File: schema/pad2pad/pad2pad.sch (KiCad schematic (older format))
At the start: 2 parts, among them J1 Conn_01x01_Male, J2 Conn_01x01_Male

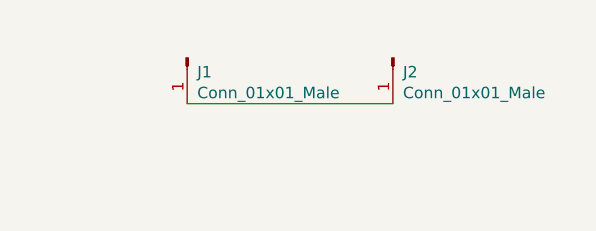
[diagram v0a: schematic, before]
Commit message: ardrill command, pad2pad&soic projects
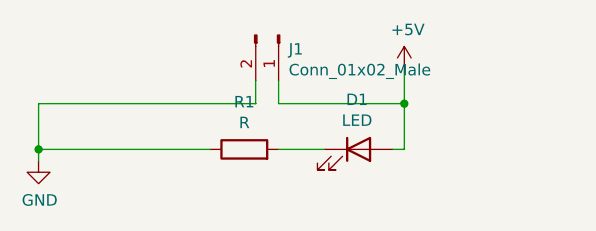
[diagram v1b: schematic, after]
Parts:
- removed J1, J2: Conn_01x01_Male, Connector_Wire:SolderWirePad_1x01_SMD_1x2mm, symbol Connector:Conn_01x01_Male
- added D1: LED, LED_SMD:LED_0805_2012Metric, symbol Device:LED
- added J1: Conn_01x02_Male, Connector_PinHeader_2.54mm:PinHeader_1x02_P2.54mm_Vertical, symbol Connector:Conn_01x02_Male
- added R1: R, Resistor_SMD:R_0805_2012Metric, symbol Device:R
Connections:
- new net: D1.1 (K), R1.2
- new net +5V: D1.2 (A), J1.1 (Pin_1)
- new net GND: J1.2 (Pin_2), R1.1
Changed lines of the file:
@@
 $EndDescr
 $Comp
-L Connector:Conn_01x01_Male J1
-U 1 1 62064621
-P 4550 1800
-F 0 "J1" V 4612 1844 50  0000 L CNN
-F 1 "Conn_01x01_Male" V 4703 1844 50  0000 L CNN
-F 2 "Connector_Wire:SolderWirePad_1x01_SMD_1x2mm" H 4550 1800 50  0001 C CNN
-F 3 "~" H 4550 1800 50  0001 C CNN
-	1    4550 1800
-	0    1    1    0
+L Device:LED D1
+U 1 1 6253249A
+P 5300 2200
+F 0 "D1" H 5293 2417 50  0000 C CNN
+F 1 "LED" H 5293 2326 50  0000 C CNN
+F 2 "LED_SMD:LED_0805_2012Metric" H 5300 2200 50  0001 C CNN
+F 3 "~" H 5300 2200 50  0001 C CNN
+	1    5300 2200
+	1    0    0    -1
 $EndComp
 $Comp
-L Connector:Conn_01x01_Male J2
-U 1 1 62064D09
-P 5450 1800
-F 0 "J2" V 5512 1844 50  0000 L CNN
-F 1 "Conn_01x01_Male" V 5603 1844 50  0000 L CNN
-F 2 "Connector_Wire:SolderWirePad_1x01_SMD_1x2mm" H 5450 1800 50  0001 C CNN
-F 3 "~" H 5450 1800 50  0001 C CNN
-	1    5450 1800
+L Device:R R1
+U 1 1 62532987
+P 4800 2200
+F 0 "R1" V 5007 2200 50  0000 C CNN
+F 1 "R" V 4916 2200 50  0000 C CNN
+F 2 "Resistor_SMD:R_0805_2012Metric" V 4730 2200 50  0001 C CNN
+F 3 "~" H 4800 2200 50  0001 C CNN
+	1    4800 2200
+	0    -1   -1   0
+$EndComp
+$Comp
+L power:+5V #PWR0101
+U 1 1 62534902
+P 5500 1850
+F 0 "#PWR0101" H 5500 1700 50  0001 C CNN
+F 1 "+5V" H 5515 2023 50  0000 C CNN
+F 2 "" H 5500 1850 50  0001 C CNN
+F 3 "" H 5500 1850 50  0001 C CNN
+	1    5500 1850
+	1    0    0    -1
+$EndComp
+$Comp
+L power:GND #PWR0102
+U 1 1 6253550C
+P 3900 2250
+F 0 "#PWR0102" H 3900 2000 50  0001 C CNN
+F 1 "GND" H 3905 2077 50  0000 C CNN
+F 2 "" H 3900 2250 50  0001 C CNN
+F 3 "" H 3900 2250 50  0001 C CNN
+	1    3900 2250
+	1    0    0    -1
+$EndComp
+Wire Wire Line
+	4650 2200 3900 2200
+Wire Wire Line
+	3900 2200 3900 2250
+Wire Wire Line
+	3900 2200 3900 2000
+Connection ~ 3900 2200
+Wire Wire Line
+	4950 2200 5150 2200
+Wire Wire Line
+	5450 2200 5500 2200
+Wire Wire Line
+	5500 2200 5500 2000
+$Comp
+L Connector:Conn_01x02_Male J1
+U 1 1 625387C7
+P 4950 1700
+F 0 "J1" V 5012 1744 50  0000 L CNN
+F 1 "Conn_01x02_Male" V 5103 1744 50  0000 L CNN
+F 2 "Connector_PinHeader_2.54mm:PinHeader_1x02_P2.54mm_Vertical" H 4950 1700 50  0001 C CNN
+F 3 "~" H 4950 1700 50  0001 C CNN
+	1    4950 1700
 	0    1    1    0
 $EndComp
 Wire Wire Line
-	4550 2000 5450 2000
+	5500 2000 4950 2000
+Wire Wire Line
+	4950 2000 4950 1900
+Connection ~ 5500 2000
+Wire Wire Line
+	3900 2000 4850 2000
+Wire Wire Line
+	4850 2000 4850 1900
+Wire Wire Line
+	5500 1850 5500 2000
 $EndSCHEMATC
